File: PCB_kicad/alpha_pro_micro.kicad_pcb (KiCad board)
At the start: 2 copper layers, 192.9 x 59.5 mm, 72 parts, among them J1 Conn_01x03, J2 Conn_01x01_Female, J3 Conn_01x01_Female, J4 Conn_01x01_Female, J5 Conn_01x01_Female, J6 Conn_01x01_Female, J7 Conn_01x01_Female, J8 Conn_01x01_Female, J9 Conn_01x01_Female, K1 KEYSW, K10 KEYSW, K11 KEYSW, K12 KEYSW, K13 KEYSW, K14 KEYSW, K15 KEYSW, K16 KEYSW, K17 KEYSW, K18 KEYSW, K19 KEYSW, K2 KEYSW, K20 KEYSW, K21 KEYSW, K22 KEYSW, K23 KEYSW, K24 KEYSW, K25 KEYSW, K26 KEYSW, K27 KEYSW, K28 KEYSW, K3 KEYSW, K4 KEYSW, K5 KEYSW, K6 KEYSW, K7 KEYSW, K8 KEYSW, K9 KEYSW, SW1 SW_Push, U1 ProMicro

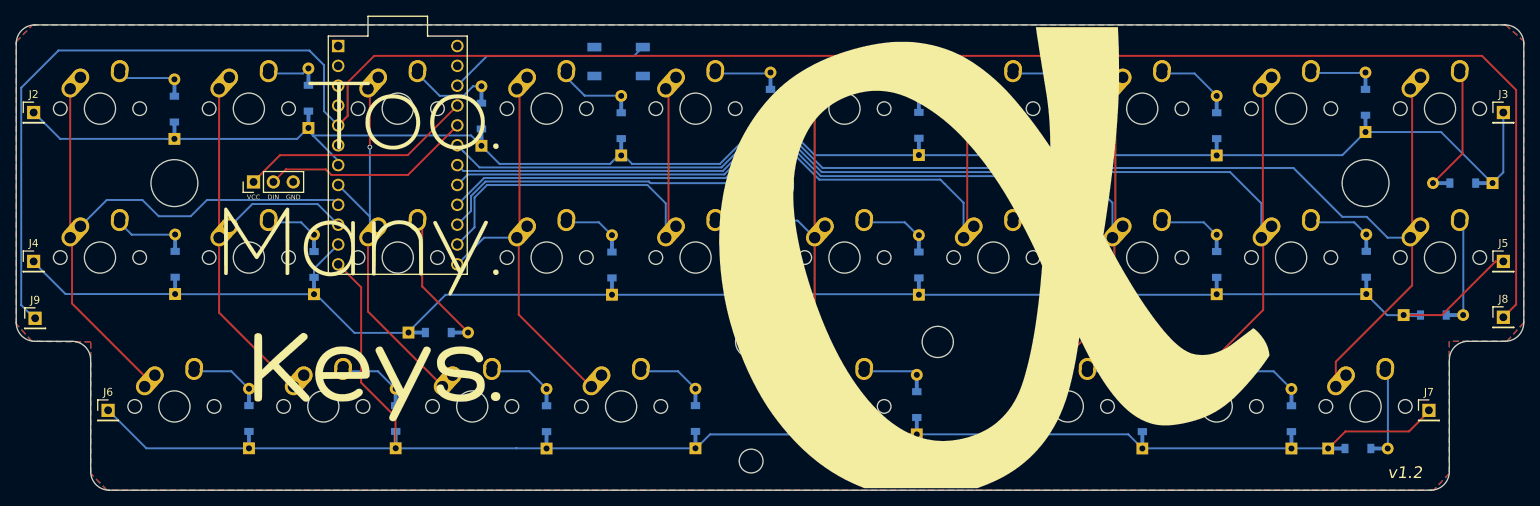
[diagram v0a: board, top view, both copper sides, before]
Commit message: Alpha v2.0 released!
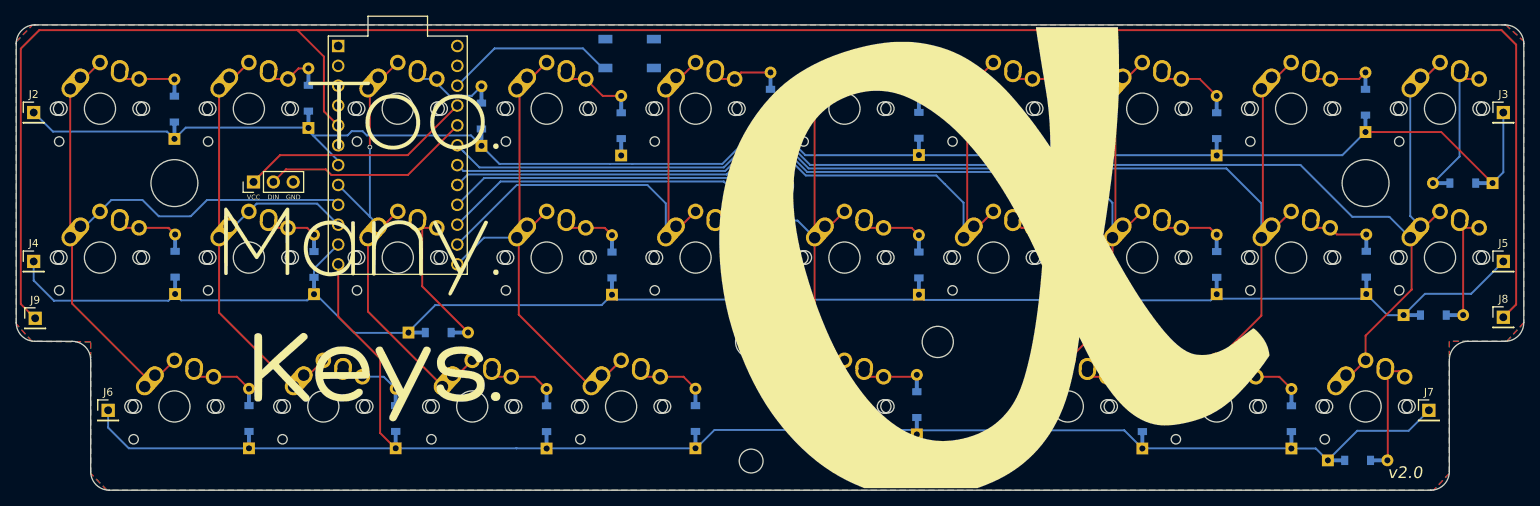
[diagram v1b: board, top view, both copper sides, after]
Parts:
- K1, K10, K11, K12, K13, K14, K15, K16, K17, K18, K19, K2, K20, K21, K22, K23, K24, K26, K27, K28, K3, K4, K5, K6, K7, K8, K9: footprint MX_Alps_Hybrid:MX-1U-NoLED -> keebio-parts:MX-Alps-Choc-1U-NoLED
- K25: footprint MX_Alps_Hybrid:MX-2U-ReversedStabilizers-NoLED -> keebio-parts:MX-Alps-Choc-2U-StabFlip
- moved SW1 1.74 mm to (144.0, 102.5), turned to 180 degrees
- moved D28 1.52 mm to (237.1, 154.5)
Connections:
- K1 pad 1: /col0 -> Net-(D1-Pad2)
- K1 pad 2: Net-(D1-Pad2) -> /col0
- K10 pad 1: /col9 -> Net-(D10-Pad2)
- K10 pad 2: Net-(D10-Pad2) -> /col9
- K11 pad 1: /col0 -> Net-(D11-Pad2)
- K11 pad 2: Net-(D11-Pad2) -> /col0
- K12 pad 1: /col1 -> Net-(D12-Pad2)
- K12 pad 2: Net-(D12-Pad2) -> /col1
- K13 pad 1: /col2 -> Net-(D13-Pad2)
- K13 pad 2: Net-(D13-Pad2) -> /col2
- K14 pad 1: /col3 -> Net-(D14-Pad2)
- K14 pad 2: Net-(D14-Pad2) -> /col3
- K15 pad 1: /col4 -> Net-(D15-Pad2)
- K15 pad 2: Net-(D15-Pad2) -> /col4
- K16 pad 1: /col5 -> Net-(D16-Pad2)
- K16 pad 2: Net-(D16-Pad2) -> /col5
- K17 pad 1: /col6 -> Net-(D17-Pad2)
- K17 pad 2: Net-(D17-Pad2) -> /col6
- K18 pad 1: /col7 -> Net-(D18-Pad2)
- K18 pad 2: Net-(D18-Pad2) -> /col7
- K19 pad 1: /col8 -> Net-(D19-Pad2)
- K19 pad 2: Net-(D19-Pad2) -> /col8
- K2 pad 1: /col1 -> Net-(D2-Pad2)
- K2 pad 2: Net-(D2-Pad2) -> /col1
- K20 pad 1: /col9 -> Net-(D20-Pad2)
- K20 pad 2: Net-(D20-Pad2) -> /col9
- K21 pad 1: /col0 -> Net-(D21-Pad2)
- K21 pad 2: Net-(D21-Pad2) -> /col0
- K22 pad 1: /col1 -> Net-(D22-Pad2)
- K22 pad 2: Net-(D22-Pad2) -> /col1
- K23 pad 1: /col2 -> Net-(D23-Pad2)
- K23 pad 2: Net-(D23-Pad2) -> /col2
- K24 pad 1: /col3 -> Net-(D24-Pad2)
- K24 pad 2: Net-(D24-Pad2) -> /col3
- K26 pad 1: /col7 -> Net-(D26-Pad2)
- K26 pad 2: Net-(D26-Pad2) -> /col7
- K27 pad 1: /col8 -> Net-(D27-Pad2)
- K27 pad 2: Net-(D27-Pad2) -> /col8
- K28 pad 1: /col9 -> Net-(D28-Pad2)
- K28 pad 2: Net-(D28-Pad2) -> /col9
- K3 pad 1: /col2 -> Net-(D3-Pad2)
- K3 pad 2: Net-(D3-Pad2) -> /col2
- K4 pad 1: /col3 -> Net-(D4-Pad2)
- K4 pad 2: Net-(D4-Pad2) -> /col3
- K5 pad 1: /col4 -> Net-(D5-Pad2)
- K5 pad 2: Net-(D5-Pad2) -> /col4
- K6 pad 1: /col5 -> Net-(D6-Pad2)
- K6 pad 2: Net-(D6-Pad2) -> /col5
- K7 pad 1: /col6 -> Net-(D7-Pad2)
- K7 pad 2: Net-(D7-Pad2) -> /col6
- K8 pad 1: /col7 -> Net-(D8-Pad2)
- K8 pad 2: Net-(D8-Pad2) -> /col7
- K9 pad 1: /col8 -> Net-(D9-Pad2)
- K9 pad 2: Net-(D9-Pad2) -> /col8
- U1 pad 1: (no net) -> Net-(U1-Pad1)
- U1 pad 2: (no net) -> Net-(U1-Pad2)
- U1 pad 24: (no net) -> Net-(U1-Pad24)
- U1 pad 6: (no net) -> Net-(U1-Pad6)
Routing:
- net /col_tmo: track 268.5 -> 278.2 mm
- net /col3: track 50.2 -> 58.9 mm
- net /col2: track 47.2 -> 55.1 mm
- net /col5: track 90.2 -> 97.7 mm
- net /row1: track 204.6 -> 210.6 mm
- net /col6: track 92.7 -> 98.1 mm
- net /col0: track 76.6 -> 81.5 mm
- net Net-(D28-Pad2): track 9.52 -> 14.3 mm
- net /col7: track 133.9 -> 138.6 mm
- net /col8: track 153.7 -> 158.2 mm
- net RST: track 25.8 -> 21.6 mm
- net /row2: track 200.9 -> 204.4 mm
- net /col4: track 55.8 -> 58.9 mm
- net Net-(D10-Pad2): track 15.2 -> 18.2 mm
- net /col9: track 171.2 -> 174.2 mm
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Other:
- board text added: "v2.0"
- board text removed: "v1.2"
